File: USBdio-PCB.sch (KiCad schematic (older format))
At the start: 68 parts, among them IC1 ATMEGA328-P, P0 RELAY_(JSM1A-12V-4), P1 RELAY_(JSM1A-12V-4), P2 RELAY_(JSM1A-12V-4), P3 RELAY_(JSM1A-12V-4), P4 RELAY_(JSM1A-12V-4), P5 RELAY_(JSM1A-12V-4), P6 RELAY_(JSM1A-12V-4), P7 RELAY_(JSM1A-12V-4), P8 CONN_01X03, Q1 Q_NPN_BEC, Q10 Q_NPN, Q11 Q_NPN, Q12 Q_NPN, Q13 Q_NPN, Q14 Q_NPN, Q15 Q_NPN, Q16 Q_NPN, Q17 Q_NPN, Q2 Q_NPN_BEC, Q3 Q_NPN_BEC, Q4 Q_NPN_BEC, Q5 Q_NPN_BEC, Q6 Q_NPN_BEC, Q7 Q_NPN_BEC, Q8 Q_NPN_BEC, Q9 Q_NPN_BEC, U1 NCV7805BDTRKG, X1 CRYSTAL_SMD

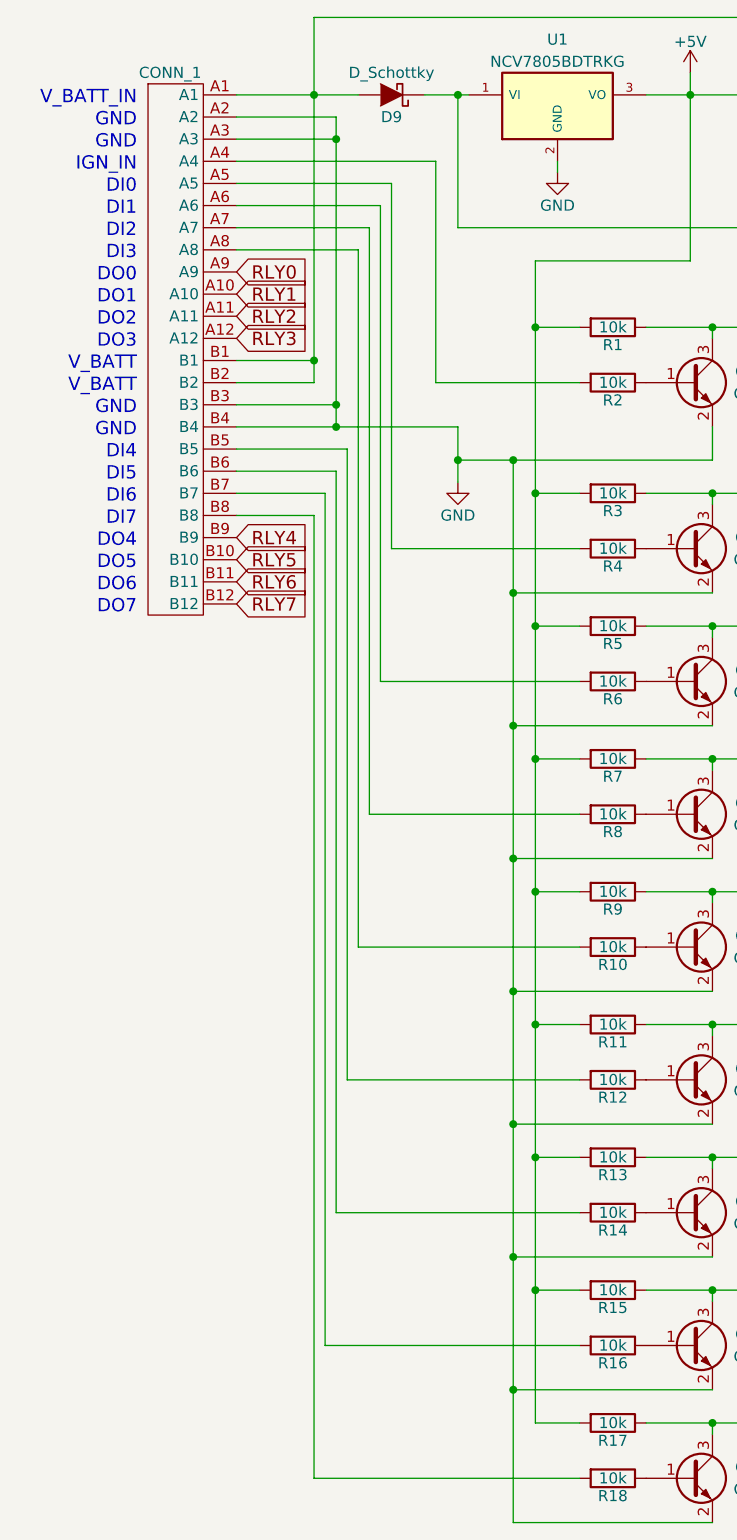
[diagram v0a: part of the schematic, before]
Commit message: almost finish with traces.
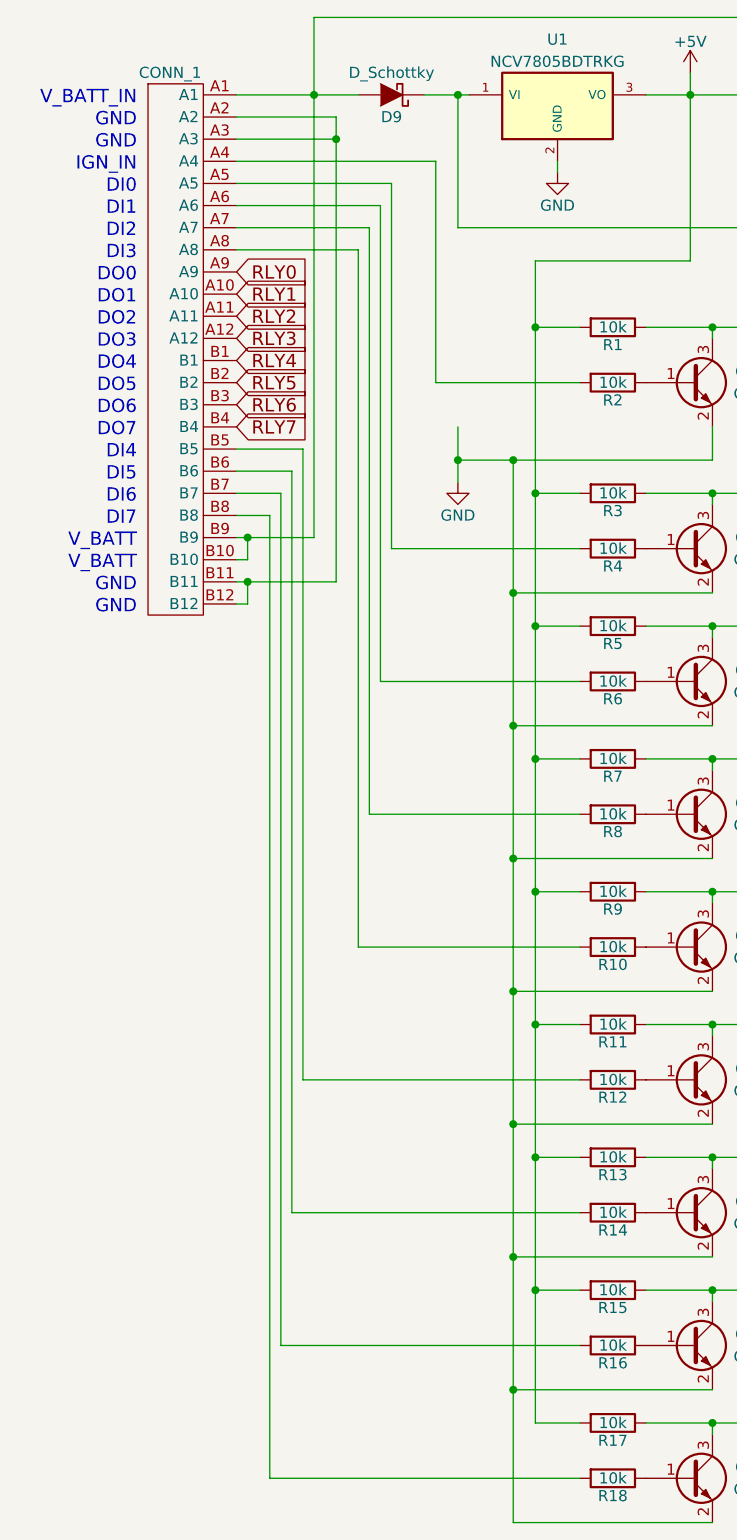
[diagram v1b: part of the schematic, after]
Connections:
- net GND: no longer CONN_1.A2, CONN_1.A3, CONN_1.B3, CONN_1.B4
- net RLY4: now also CONN_1.B1; no longer CONN_1.B9
- net RLY5: now also CONN_1.B2; no longer CONN_1.B10
- net RLY6: now also CONN_1.B3; no longer CONN_1.B11
- net RLY7: now also CONN_1.B4; no longer CONN_1.B12
- net at CONN_1.A1, D9.2 (A), P0.1 (POLE)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: now also CONN_1.B10, CONN_1.B9; no longer CONN_1.B1, CONN_1.B2
- new net: CONN_1.A2, CONN_1.A3, CONN_1.B11, CONN_1.B12
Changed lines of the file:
@@
 Text Notes 1300 2900 2    60   ~ 0
 DI7
+Text Notes 1300 2200 2    60   ~ 0
+DO4
+Text Notes 1300 2300 2    60   ~ 0
+DO5
+Text Notes 1300 2400 2    60   ~ 0
+DO6
+Text Notes 1300 2500 2    60   ~ 0
+DO7
+Text Notes 1300 3300 2    60   ~ 0
+GND
+Text Notes 1300 3200 2    60   ~ 0
+GND
 Text Notes 1300 3000 2    60   ~ 0
-DO4
+V_BATT
 Text Notes 1300 3100 2    60   ~ 0
-DO5
-Text Notes 1300 3200 2    60   ~ 0
-DO6
-Text Notes 1300 3300 2    60   ~ 0
-DO7
-Text Notes 1300 2500 2    60   ~ 0
-GND
-Text Notes 1300 2400 2    60   ~ 0
-GND
-Text Notes 1300 2200 2    60   ~ 0
-V_BATT
-Text Notes 1300 2300 2    60   ~ 0
 V_BATT
 $Comp
@@
 Text GLabel 1750 2050 2    60   Input ~ 0
 RLY3
-Text GLabel 1750 2950 2    60   Input ~ 0
+Text GLabel 1750 2150 2    60   Input ~ 0
 RLY4
-Text GLabel 1750 3050 2    60   Input ~ 0
+Text GLabel 1750 2250 2    60   Input ~ 0
 RLY5
-Text GLabel 1750 3150 2    60   Input ~ 0
+Text GLabel 1750 2350 2    60   Input ~ 0
 RLY6
-Text GLabel 1750 3250 2    60   Input ~ 0
+Text GLabel 1750 2450 2    60   Input ~ 0
 RLY7
 Wire Wire Line
@@
 Connection ~ 3100 6350
 Wire Wire Line
-	2250 5400 3300 5400
-Wire Wire Line
-	2200 6000 3300 6000
-Wire Wire Line
-	2150 6600 3300 6600
-Wire Wire Line
-	2100 7200 3300 7200
+	2050 5400 3300 5400
+Wire Wire Line
+	2000 6000 3300 6000
+Wire Wire Line
+	1950 6600 3300 6600
+Wire Wire Line
+	1900 7200 3300 7200
 Wire Wire Line
 	3900 2600 3900 2450
@@
 	9050 600  2100 600
 Wire Wire Line
-	2100 600  2100 2250
+	2100 600  2100 2950
 Connection ~ 2100 950
 Wire Wire Line
@@
 	2300 4800 3300 4800
 Wire Wire Line
-	1750 2550 2250 2550
-Wire Wire Line
-	2250 2550 2250 5400
-Wire Wire Line
-	2200 6000 2200 2650
-Wire Wire Line
-	2200 2650 1750 2650
-Wire Wire Line
-	1750 2750 2150 2750
-Wire Wire Line
-	2150 2750 2150 6600
-Wire Wire Line
-	2100 7200 2100 2850
-Wire Wire Line
-	2100 2850 1750 2850
+	1750 2550 2050 2550
+Wire Wire Line
+	2050 2550 2050 5400
+Wire Wire Line
+	2000 6000 2000 2650
+Wire Wire Line
+	2000 2650 1750 2650
+Wire Wire Line
+	1750 2750 1950 2750
+Wire Wire Line
+	1950 2750 1950 6600
+Wire Wire Line
+	1900 7200 1900 2850
+Wire Wire Line
+	1900 2850 1750 2850
 Wire Wire Line
 	2750 2450 2750 2700
-Wire Wire Line
-	1750 2450 2750 2450
 Connection ~ 2750 2600
 Wire Wire Line
 	1750 1050 2200 1050
 Wire Wire Line
-	2200 1050 2200 2450
-Connection ~ 2200 2450
-Wire Wire Line
-	1750 2350 2200 2350
-Connection ~ 2200 2350
+	2200 1050 2200 3150
 Wire Wire Line
 	1750 1150 2200 1150
@@
 	2750 1550 2750 950
 Connection ~ 2750 950
-Wire Wire Line
-	2100 2250 1750 2250
-Wire Wire Line
-	1750 2150 2100 2150
-Connection ~ 2100 2150
 $Comp
 L RELAY_(JSM1A-12V-4) P7
@@
 Wire Wire Line
 	7350 5450 7350 4850
+Wire Wire Line
+	2100 2950 1750 2950
+Wire Wire Line
+	1750 3050 1800 3050
+Wire Wire Line
+	1800 3050 1800 2950
+Connection ~ 1800 2950
+Wire Wire Line
+	2200 3150 1750 3150
+Wire Wire Line
+	1750 3250 1800 3250
+Wire Wire Line
+	1800 3250 1800 3150
+Connection ~ 1800 3150
 $EndSCHEMATC

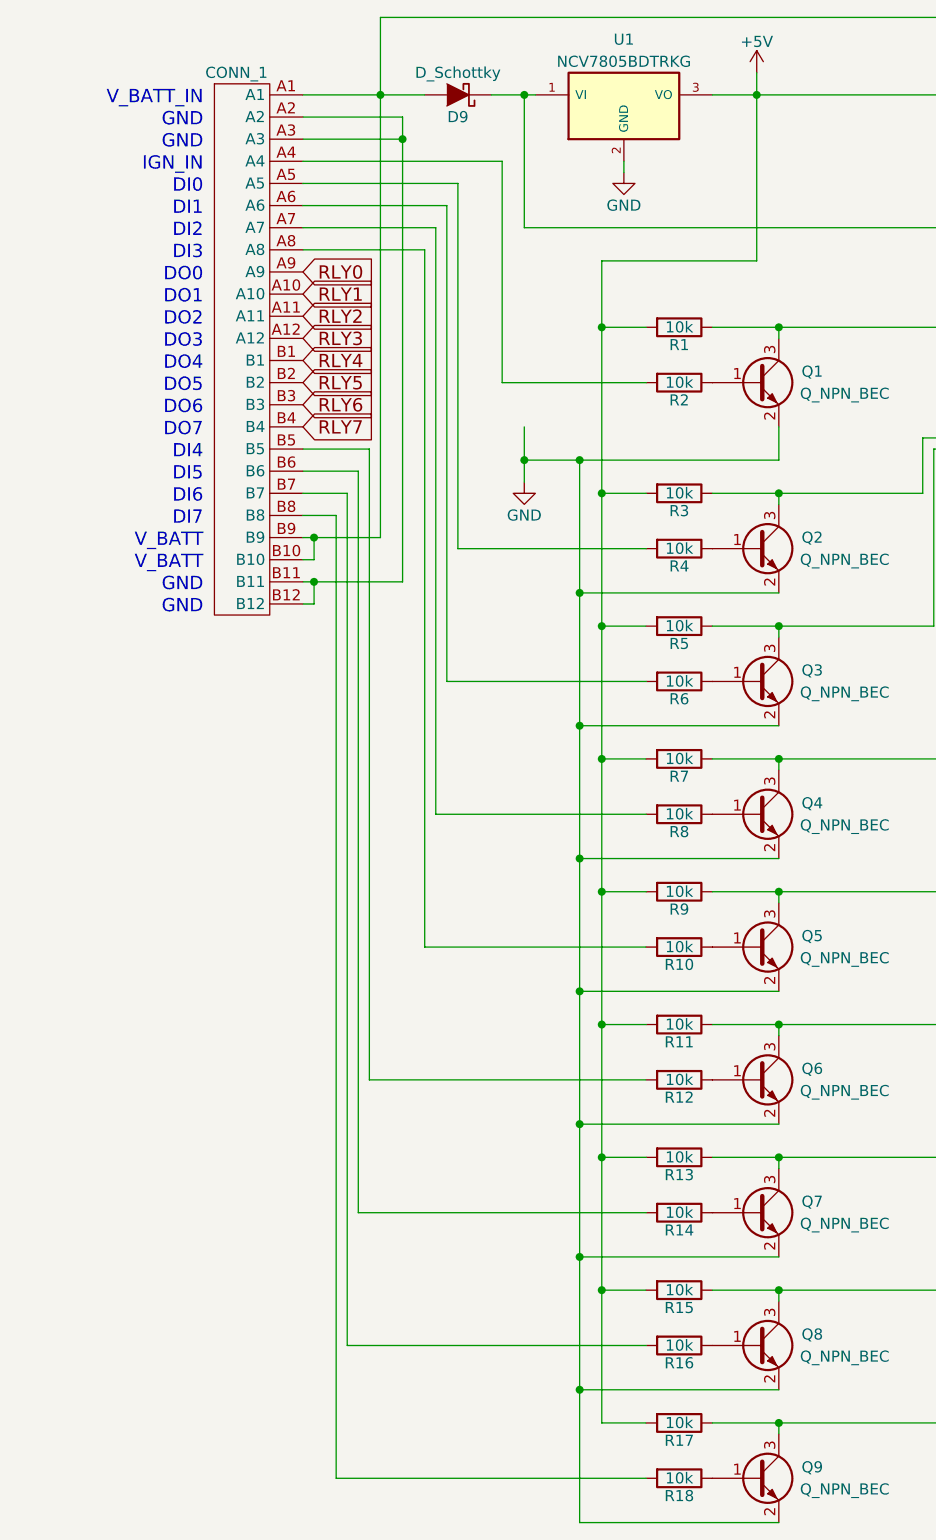
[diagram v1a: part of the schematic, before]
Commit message: finished traces
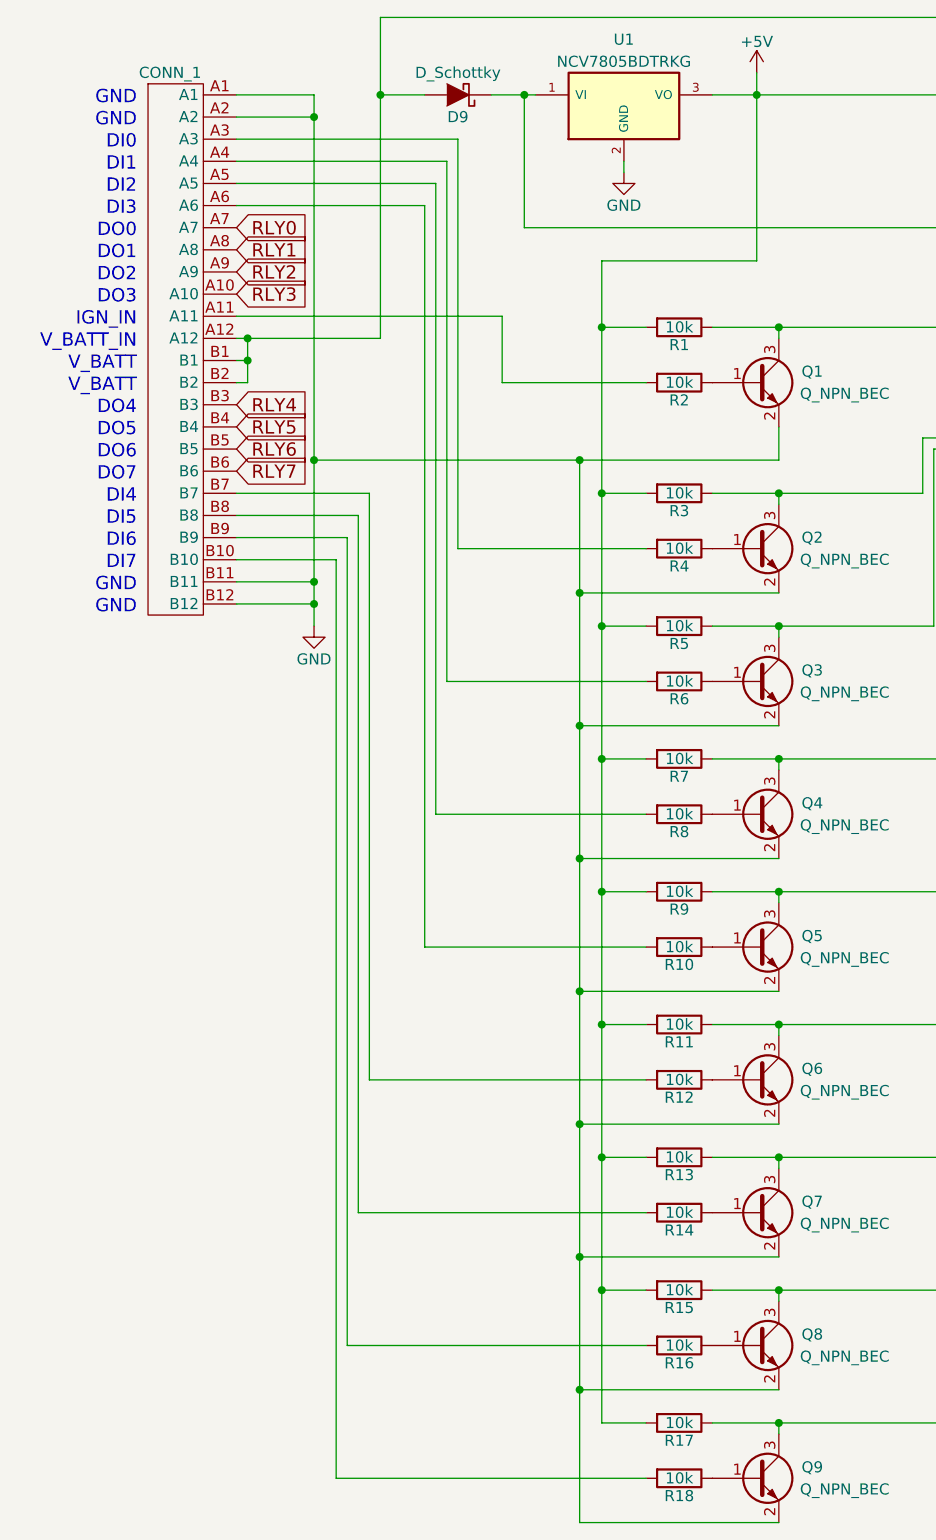
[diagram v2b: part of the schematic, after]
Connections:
- net GND: now also CONN_1.A1, CONN_1.A2, CONN_1.B11, CONN_1.B12
- net RLY0: now also CONN_1.A7; no longer CONN_1.A9
- net RLY1: now also CONN_1.A8; no longer CONN_1.A10
- net RLY2: now also CONN_1.A9; no longer CONN_1.A11
- net RLY3: now also CONN_1.A10; no longer CONN_1.A12
- net RLY4: now also CONN_1.B3; no longer CONN_1.B1
- net RLY5: now also CONN_1.B4; no longer CONN_1.B2
- net RLY6: now also CONN_1.B5; no longer CONN_1.B3
- net RLY7: now also CONN_1.B6; no longer CONN_1.B4
- net at R4.2: now also CONN_1.A3; no longer CONN_1.A5
- net at R6.2: now also CONN_1.A4; no longer CONN_1.A6
- net at R8.2: now also CONN_1.A5; no longer CONN_1.A7
- net at R10.2: now also CONN_1.A6; no longer CONN_1.A8
- net at R12.2: now also CONN_1.B7; no longer CONN_1.B5
- net at R14.2: now also CONN_1.B8; no longer CONN_1.B6
- net at R16.2: now also CONN_1.B9; no longer CONN_1.B7
- net at R18.2: now also CONN_1.B10; no longer CONN_1.B8
- net at R2.2: now also CONN_1.A11; no longer CONN_1.A4
- net at D9.2 (A), P0.1 (POLE), P1.1 (POLE)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: now also CONN_1.A12, CONN_1.B1, CONN_1.B2; no longer CONN_1.A1, CONN_1.B10, CONN_1.B9
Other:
- moved on the sheet: CONN_1
